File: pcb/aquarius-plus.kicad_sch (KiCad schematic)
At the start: 216 parts, among them J1 Cassette in, J10 Audio out, J11 Hand controller 2, J12 ESP USB Host, J13 Power in, J14 FPGA spare, J15 Expansion port, J16 ESP32 spare, J2 Cassette out, J3 SD_Card, J4 Printer, J5 Hand controller 1, J6 VGA, J7 DBG, J8 USB_A, J9 USB_A, Q1 BC847C, Q2 BC847C, SW1 SW_DPDT_x2, U1 XC3S200-4TQG144, U10 IS61C5128AS-25QLI, U11 74LVC4245APW, U12 74HC166, U13 SST39SF020A-55-4C-WHE, U14 74LVC4245APW, U15 LDL1117S33R, U16 MCP1700T-2502E/TT, U17 LD1117S12, U2 SN74CBTD3861PWR, U3 MAX3221ECPWR, U4 SN74CBTD3861PWR, U5 ESP32-S2-SOLO-N4R2, U6 SN74CBTD3861PWR, U7 Z84C0010AEG, U8 SN74CBTD3861PWR, U9 74HC166, X1 SG-5032CAN, X2 SG-5032CAN

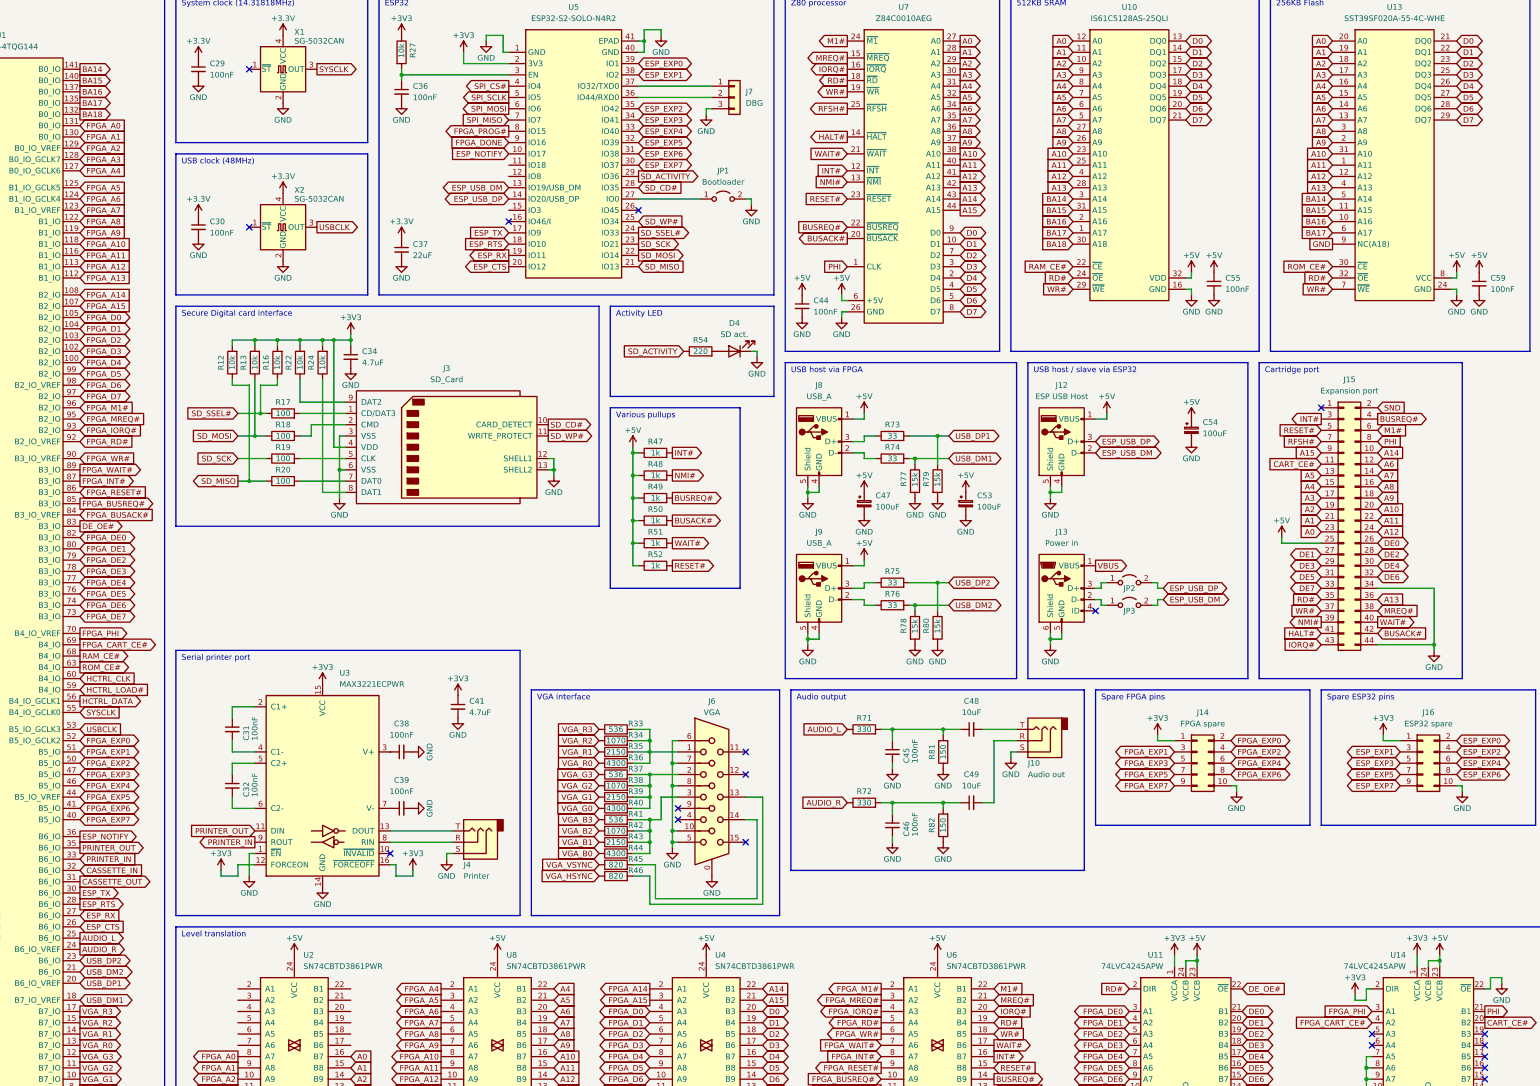
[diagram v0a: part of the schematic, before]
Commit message: Working on layout.
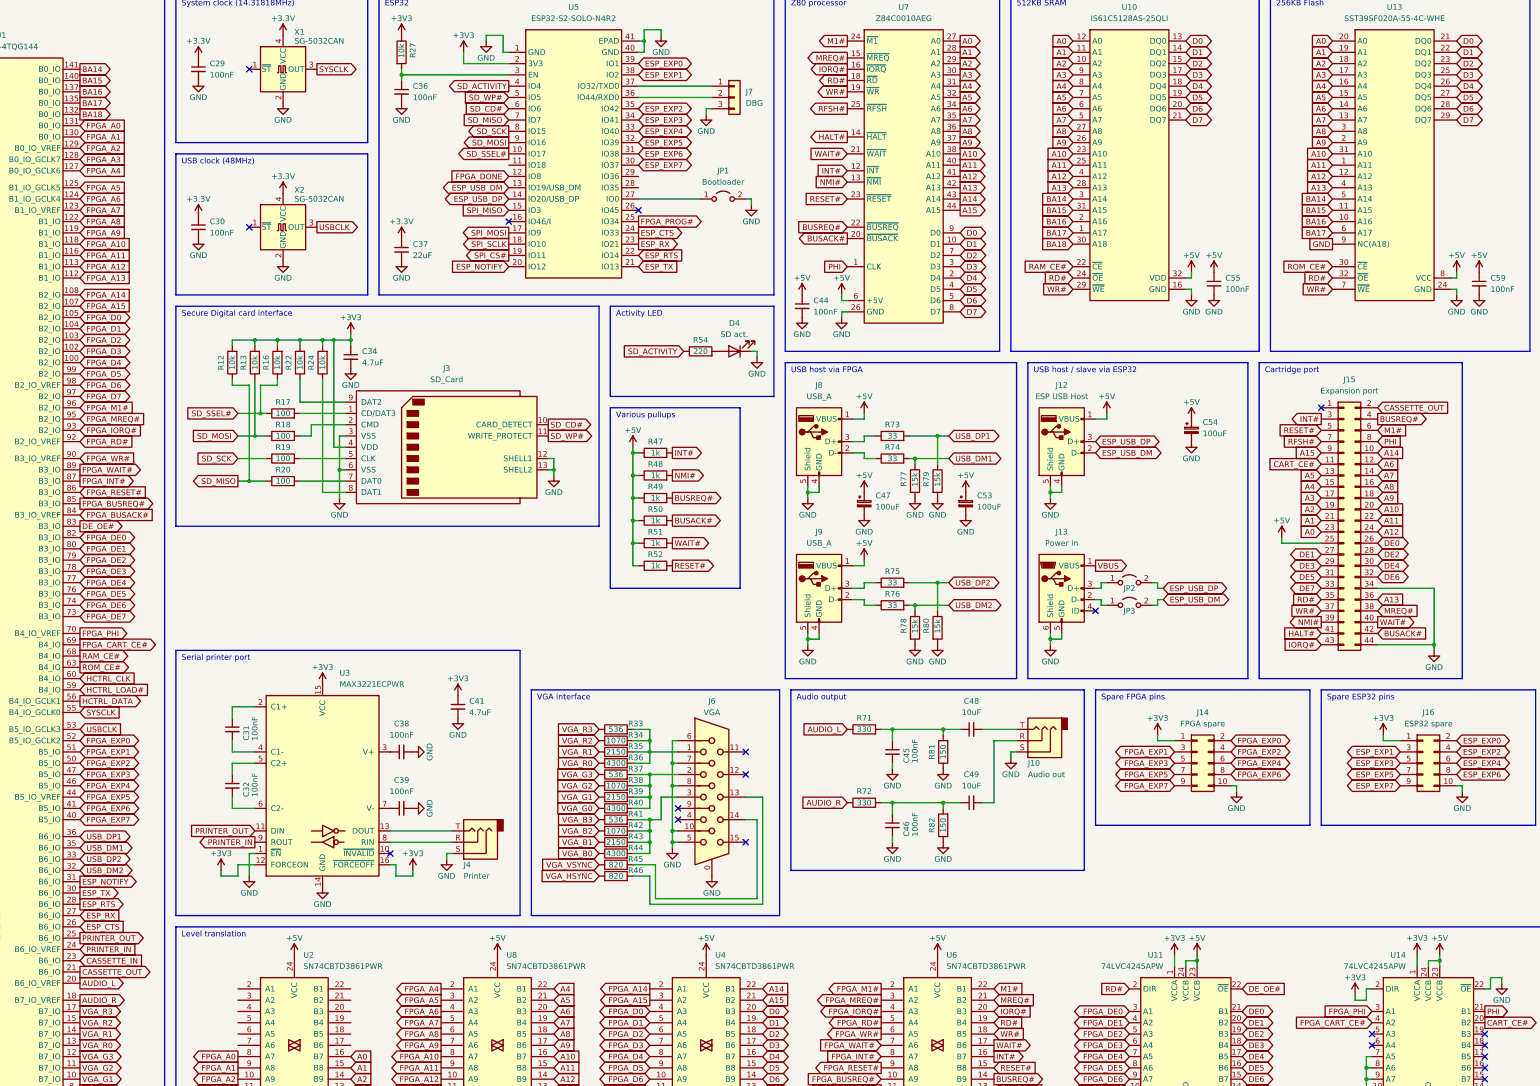
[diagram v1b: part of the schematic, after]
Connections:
- net SND is gone; now on net CASSETTE_OUT: J15.2 (Pin_2)
- net AUDIO_L: now also U1.20 (B6_IO_VREF); no longer U1.25 (B6_IO)
- net AUDIO_R: now also U1.18 (B7_IO_VREF); no longer U1.24 (B6_IO_VREF)
- net CASSETTE_IN: now also U1.23 (B6_IO); no longer U1.32 (B6_IO)
- net CASSETTE_OUT: now also U1.21 (B6_IO); no longer U1.31 (B6_IO)
- net ESP_CTS: now also U5.24 (IO33); no longer U5.20 (IO12)
- net ESP_NOTIFY: now also U1.31 (B6_IO), U5.20 (IO12); no longer U1.36 (B6_IO), U5.10 (IO17)
- net ESP_RTS: now also U5.22 (IO14); no longer U5.18 (IO10)
- net ESP_RX: now also U5.23 (IO21); no longer U5.19 (IO11)
- net ESP_TX: now also U5.21 (IO13); no longer U5.17 (IO9)
- net FPGA_DONE: now also U5.12 (IO8); no longer U5.9 (IO16)
- net FPGA_PROG#: now also U5.25 (IO34); no longer U5.8 (IO15)
- net PRINTER_IN: now also U1.24 (B6_IO_VREF); no longer U1.33 (B6_IO)
- net PRINTER_OUT: now also U1.25 (B6_IO); no longer U1.35 (B6_IO)
- net SD_ACTIVITY: now also U5.4 (IO4); no longer U5.29 (IO36)
- net SD_CD#: now also U5.6 (IO6); no longer U5.28 (IO35)
- net SD_MISO: now also U5.7 (IO7); no longer U5.21 (IO13)
- net SD_MOSI: now also U5.9 (IO16); no longer U5.22 (IO14)
- net SD_SCK: now also U5.8 (IO15); no longer U5.23 (IO21)
- net SD_SSEL#: now also U5.10 (IO17); no longer U5.24 (IO33)
- net SD_WP#: now also U5.5 (IO5); no longer U5.25 (IO34)
- net SPI_CS#: now also U5.19 (IO11); no longer U5.4 (IO4)
- net SPI_MISO: now also U5.15 (IO3); no longer U5.7 (IO7)
- net SPI_MOSI: now also U5.17 (IO9); no longer U5.6 (IO6)
- net SPI_SCLK: now also U5.18 (IO10); no longer U5.5 (IO5)
- net USB_DM1: now also U1.35 (B6_IO); no longer U1.18 (B7_IO_VREF)
- net USB_DM2: now also U1.32 (B6_IO); no longer U1.21 (B6_IO)
- net USB_DP1: now also U1.36 (B6_IO); no longer U1.20 (B6_IO_VREF)
- net USB_DP2: now also U1.33 (B6_IO); no longer U1.23 (B6_IO)
